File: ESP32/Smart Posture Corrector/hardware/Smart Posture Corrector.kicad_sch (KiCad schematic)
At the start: 0 parts

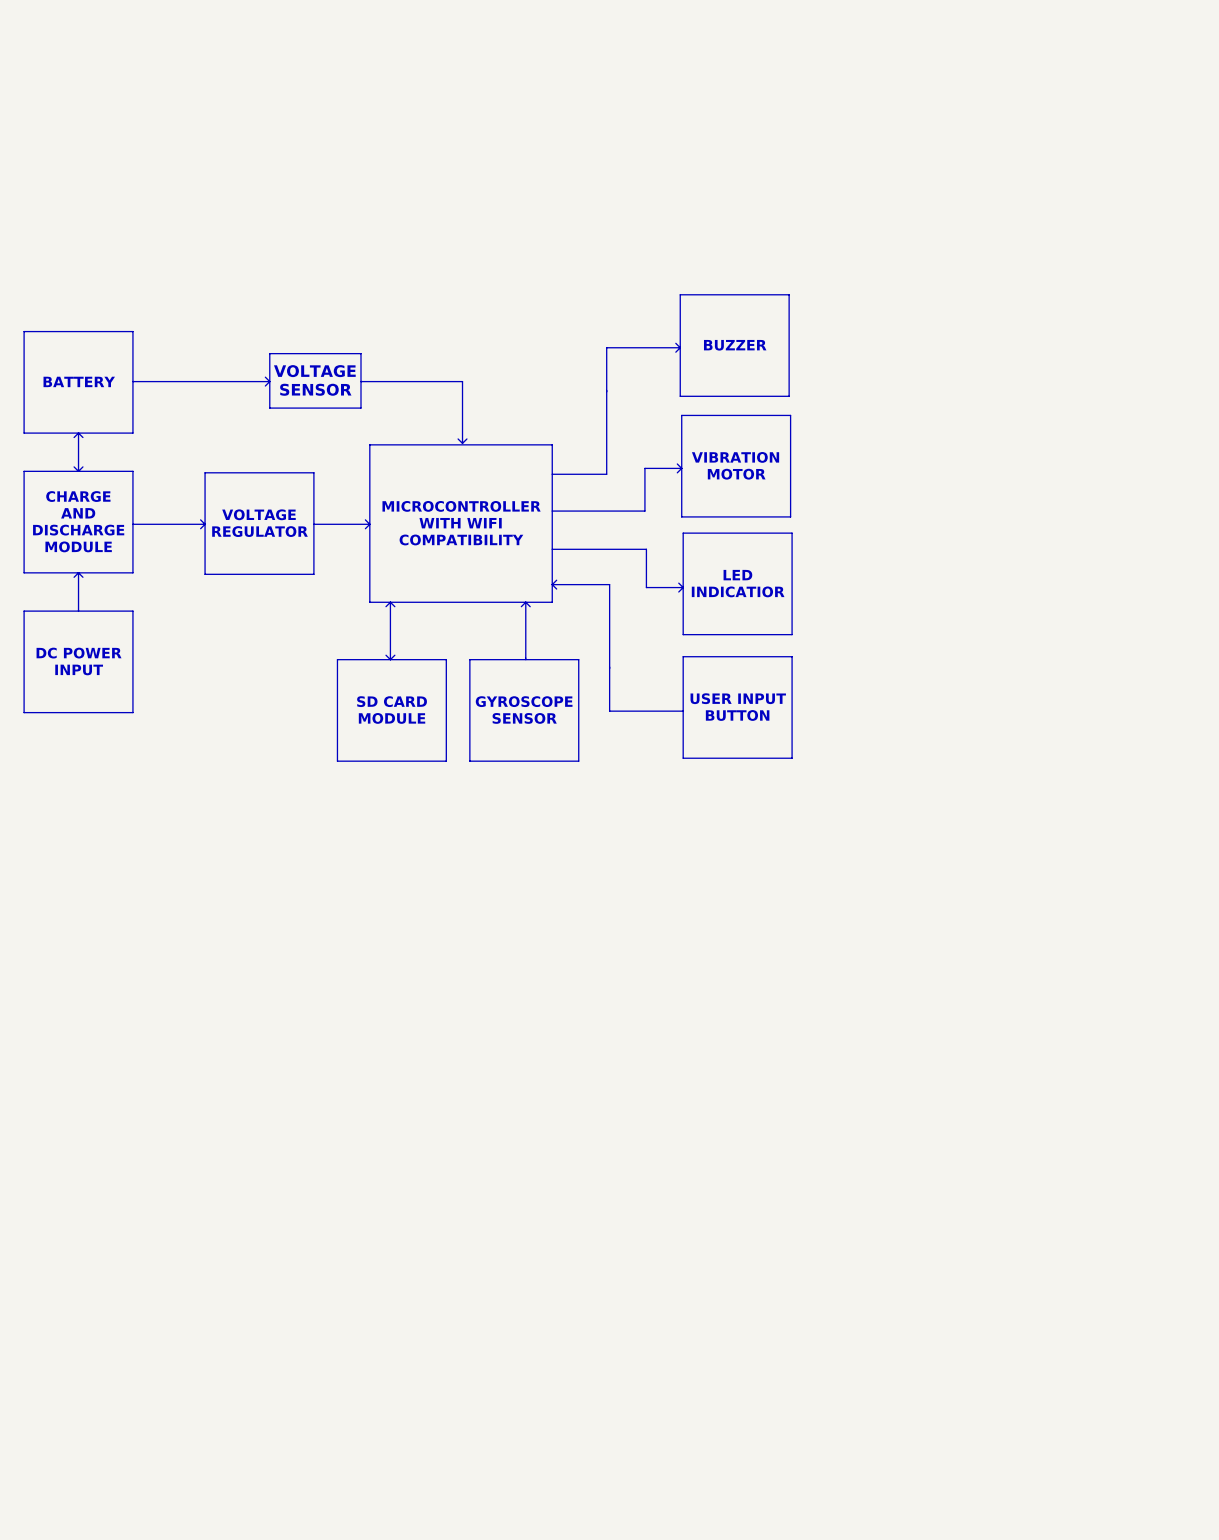
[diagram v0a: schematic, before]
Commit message: Schematic in making
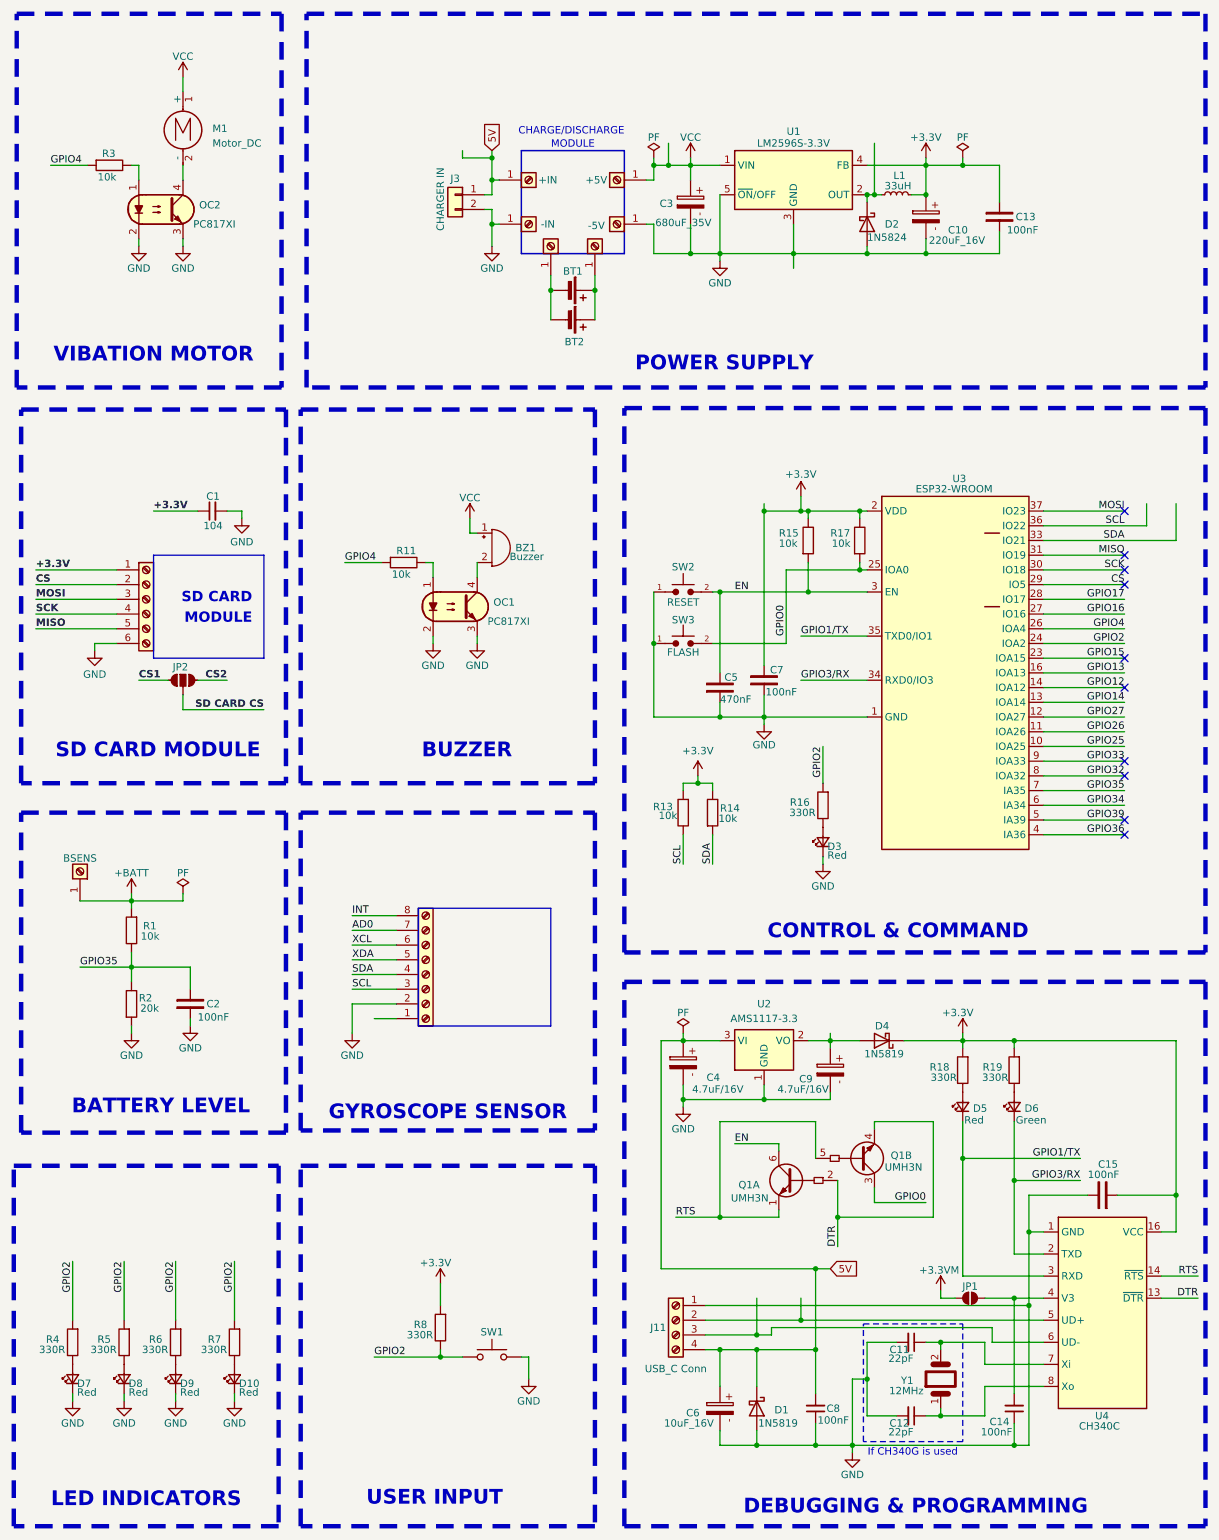
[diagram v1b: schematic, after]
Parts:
- added BT1, BT2: Battery_Cell, symbol Device:Battery_Cell
- added BZ1: Buzzer, Buzzer_Beeper:Buzzer_15x7.5RM7.6, symbol Device:Buzzer
- added C1: 104, Capacitor_SMD:C_0805_2012Metric, symbol Device:C_Small
- added C10: 220uF_16V, Capacitor_SMD:CP_Elec_6.3x7.7, symbol PCM_SL_Capacitors:470uF_35V
- added C11, C12: 22pF, Capacitor_SMD:C_0805_2012Metric_Pad1.18x1.45mm_HandSolder, symbol Device:C_Small
- added C13, C15, C2, C7: 100nF, Capacitor_SMD:C_0805_2012Metric_Pad1.18x1.45mm_HandSolder, symbol PCM_SL_Capacitors:104_Ceramic
- added C14, C8: 100nF, Capacitor_SMD:C_0805_2012Metric_Pad1.18x1.45mm_HandSolder, symbol Device:C_Small
- added C3: 680uF_35V, Capacitor_SMD:CP_Elec_10x12.5, symbol PCM_SL_Capacitors:470uF_35V
- added C4, C9: 4.7uF/16V, Capacitor_Tantalum_SMD:CP_EIA-3528-21_Kemet-B_HandSolder, symbol PCM_SL_Capacitors:4.7uF_16V
- added C5: 470nF, Capacitor_SMD:C_0805_2012Metric_Pad1.18x1.45mm_HandSolder, symbol PCM_SL_Capacitors:104_Ceramic
- added C6: 10uF_16V, Capacitor_THT:CP_Radial_D5.0mm_P2.00mm, symbol PCM_SL_Capacitors:10uF_16V
- added D1, D4: 1N5819, Diode_SMD:D_SMA, symbol Diode:1N5819
- added D10, D3, D5, D7, D8, D9: Red, LED_THT:LED_D3.0mm, symbol SparkFun-LED:LED_Red_0603
- added D2: 1N5824, Diode_SMD:D_SMA, symbol Diode:1N5822
- added D6: Green, LED_THT:LED_D3.0mm, symbol SparkFun-LED:LED_Red_0603
- added J1: MPU6050, symbol Connector:Screw_Terminal_01x08
- added J10: -5V, TestPoint:TestPoint_Keystone_5015_Micro_Mini, symbol Connector:Screw_Terminal_01x01
- added J11: USB_C Conn, Connector_PinHeader_2.54mm:PinHeader_1x04_P2.54mm_Vertical, symbol Connector:Screw_Terminal_01x04
- added J15: SD MODULE, Connector_PinHeader_2.54mm:PinHeader_1x06_P2.54mm_Vertical, symbol Connector:Screw_Terminal_01x06
- added J24: BSENS, Connector_Wire:SolderWire-0.1sqmm_1x01_D0.4mm_OD1mm, symbol Connector:Screw_Terminal_01x01
- added J3: CHARGER IN, symbol Connector_Generic:Conn_01x02
- added J5: +IN, TestPoint:TestPoint_Keystone_5015_Micro_Mini, symbol Connector:Screw_Terminal_01x01
- added J6: -IN, TestPoint:TestPoint_Keystone_5015_Micro_Mini, symbol Connector:Screw_Terminal_01x01
- added J7: -BATT, symbol Connector:Screw_Terminal_01x01
- added J8: +BATT, symbol Connector:Screw_Terminal_01x01
- added J9: +5V, TestPoint:TestPoint_Keystone_5015_Micro_Mini, symbol Connector:Screw_Terminal_01x01
- added JP1: ~, Jumper:SolderJumper-2_P1.3mm_Open_Pad1.0x1.5mm, symbol SparkFun-Jumper:SolderJumper_2_Open
- added JP2: ~, Jumper:SolderJumper-3_P1.3mm_Open_Pad1.0x1.5mm, symbol PCM_SparkFun-Jumper:SolderJumper_3_Open
- added L1: 33uH, Inductor_SMD:L_12x12mm_H6mm, symbol Device:L_Small
- added M1: Motor_DC, symbol Motor:Motor_DC
- added OC1, OC2: PC817XI, PCM_Package_DIP_AKL:SMDIP-4_W9.53mm, symbol PCM_Optocoupler_AKL:PC817XI
- added Q1: UMH3N, Package_TO_SOT_SMD:SOT-363_SC-70-6, symbol Transistor_BJT:UMH3N
- added R1, R11, R13, R14, R15, R17, R3: 10k, Resistor_SMD:R_0805_2012Metric, symbol PCM_SL_Resistors:10k
- added R16, R18, R19, R4, R5, R6, R7, R8: 330R, Resistor_SMD:R_0805_2012Metric, symbol PCM_SL_Resistors:1M
- added R2: 20k, Resistor_SMD:R_0805_2012Metric, symbol PCM_SL_Resistors:10k
- added SW1: SW_Push, symbol Switch:SW_Push
- added SW2: RESET, Button_Switch_SMD:SW_SPST_CK_KXT3, symbol PCM_SL_Devices:Push_Button
- added SW3: FLASH, Button_Switch_SMD:SW_SPST_CK_KXT3, symbol PCM_SL_Devices:Push_Button
- added U1: LM2596S-3.3V, Package_TO_SOT_SMD:TO-263-5_TabPin6, symbol Regulator_Switching:LM2596S-3.3
- added U2: AMS1117-3.3, Package_TO_SOT_SMD:SOT-223-3_TabPin2, symbol Regulator_Linear:AMS1117-3.3
- added U3: ESP32-WROOM, RF_Module:ESP32-WROOM-32U, symbol SparkFun-RF:ESP32-WROOM
- added U4: CH340C, Package_SO:SOIC-16_3.9x9.9mm_P1.27mm, symbol Interface_USB:CH340C
- added Y1: 12MHz, Crystal:Crystal_HC49-4H_Vertical, symbol PCM_SL_Devices:Crystal_16MHz
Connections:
- new net: C14.2, JP1.1 (A), U4.4 (V3)
- new net: J11.2 (Pin_2), U4.5 (UD+)
- new net: J11.3 (Pin_3), U4.6 (UD-)
- new net: C11.1, U4.7 (Xi), Y1.2
- new net: C12.1, U4.8 (Xo), Y1.1
- new net: OC1.1, R11.2
- new net: D5.2 (A), R18.2
- new net: D9.2 (A), R6.2
- new net: BT1.1 (+), BT2.1 (+), J8.1 (Pin_1)
- new net: C9.1, D4.2 (A), U2.2 (VO)
- new net: D3.2 (A), R16.2
- new net: D8.2 (A), R5.2
- new net: D2.1 (K), L1.1, U1.2 (OUT)
- new net: OC2.1, R3.2
- new net: M1.2 (-), OC2.4
- new net: D7.2 (A), R4.2
- new net: BT1.2 (-), BT2.2 (-), J7.1 (Pin_1)
- new net: BZ1.2 (-), OC1.4
- new net: D10.2 (A), R7.2
- new net: D6.2 (A), R19.2
- new net +3.3V: C1.1, C10.1, C13.2, C15.1, C7.2, D4.1 (K), J15.1 (Pin_1), L1.2, R13.1, R14.2, R15.2, R17.2, R18.1, R19.1, R8.1, U1.4 (FB), U3.2 (VDD), U4.16 (VCC)
- new net +3.3VM: JP1.2 (B)
- new net +BATT: J24.1 (Pin_1), R1.1
- new net 5V: C4.1, C6.1, C8.2, D1.1 (K), J11.4 (Pin_4), J3.1 (Pin_1), J5.1 (Pin_1), U2.3 (VI)
- new net AD0: J1.7 (Pin_7)
- new net CS: J15.2 (Pin_2), U3.29 (IO5)
- new net CS1: JP2.1 (A)
- new net CS2: JP2.3 (C)
- new net DTR: Q1.2 (B1), Q1.4 (E2), U4.13 (~{DTR})
- new net EN: C5.2, Q1.6 (C1), R15.1, SW2.2, U3.3 (EN)
- new net GND: C1.2, C10.2, C11.2, C12.2, C13.1, C14.1, C15.2, C2.1, C3.2, C4.2, C5.1, C6.2, C7.1, C8.1, C9.2, D1.2 (A), D10.1 (K), D2.2 (A), D3.1 (K), D7.1 (K), D8.1 (K), D9.1 (K), J1.2 (Pin_2), J10.1 (Pin_1), J11.1 (Pin_1), J15.6 (Pin_6), J3.2 (Pin_2), J6.1 (Pin_1), OC1.2, OC1.3, OC2.2, OC2.3, R2.1, SW1.2, SW2.1, SW3.1, U1.3 (GND), U1.5 (~{ON}/OFF), U1.6 (GND), U2.1 (GND), U3.1 (GND), U3.15 (GND), U3.38 (GND), U3.39 (GND), U4.1 (GND)
- new net GPIO0: Q1.3 (C2), R17.1, SW3.2, U3.25 (IOA0)
- new net GPIO12: U3.14 (IOA12)
- new net GPIO13: U3.16 (IOA13)
- new net GPIO14: U3.13 (IOA14)
- new net GPIO15: U3.23 (IOA15)
- new net GPIO16: U3.27 (IO16)
- new net GPIO17: U3.28 (IO17)
- new net GPIO1/TX: D5.1 (K), U3.35 (TXD0/IO1), U4.3 (RXD)
- new net GPIO2: R16.1, R4.1, R5.1, R6.1, R7.1, R8.2, SW1.1, U3.24 (IOA2)
- new net GPIO25: U3.10 (IOA25)
- new net GPIO26: U3.11 (IOA26)
- new net GPIO27: U3.12 (IOA27)
- new net GPIO32: U3.8 (IOA32)
- new net GPIO33: U3.9 (IOA33)
- new net GPIO34: U3.6 (IA34)
- new net GPIO35: C2.2, R1.2, R2.2, U3.7 (IA35)
- new net GPIO36: U3.4 (IA36)
- new net GPIO39: U3.5 (IA39)
- new net GPIO3/RX: D6.1 (K), U3.34 (RXD0/IO3), U4.2 (TXD)
- new net GPIO4: R11.1, R3.1, U3.26 (IOA4)
- new net INT: J1.8 (Pin_8)
- new net MISO: J15.5 (Pin_5), U3.31 (IO19)
- new net MOSI: J15.3 (Pin_3), U3.37 (IO23)
- new net RTS: Q1.1 (E1), Q1.5 (B2), U4.14 (~{RTS})
- new net SCK: J15.4 (Pin_4), U3.30 (IO18)
- new net SCL: J1.3 (Pin_3), R13.2, U3.36 (IO22)
- new net SD CARD CS: JP2.2 (B)
- new net SDA: J1.4 (Pin_4), R14.1, U3.33 (IO21)
- new net VCC: BZ1.1 (+), C3.1, J9.1 (Pin_1), M1.1 (+), U1.1 (VIN)
- new net XCL: J1.6 (Pin_6)
- new net XDA: J1.5 (Pin_5)
- no-connect marks 0 -> 10
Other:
- note added: "BATTERY LEVEL"
- note added: "BUZZER"
- note added: "CHARGE/DISCHARGE"
- note added: "CONTROL & COMMAND"
- note added: "DEBUGGING & PROGRAMMING"
- note added: "GYROSCOPE SENSOR"
- note added: "If CH340G is used"
- note added: "LED INDICATORS"
- note added: "MODULE"
- note added: "POWER SUPPLY"
- note added: "SD CARD"
- note added: "SD CARD MODULE"
- note added: "USER INPUT"
- note added: "VIBATION MOTOR"
